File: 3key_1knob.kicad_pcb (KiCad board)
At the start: 2 copper layers, 17 parts, among them SW1 RotaryEncoder_Switch, U4 Kailh_socket_MX, U5 Kailh_socket_MX, U6 Kailh_socket_MX

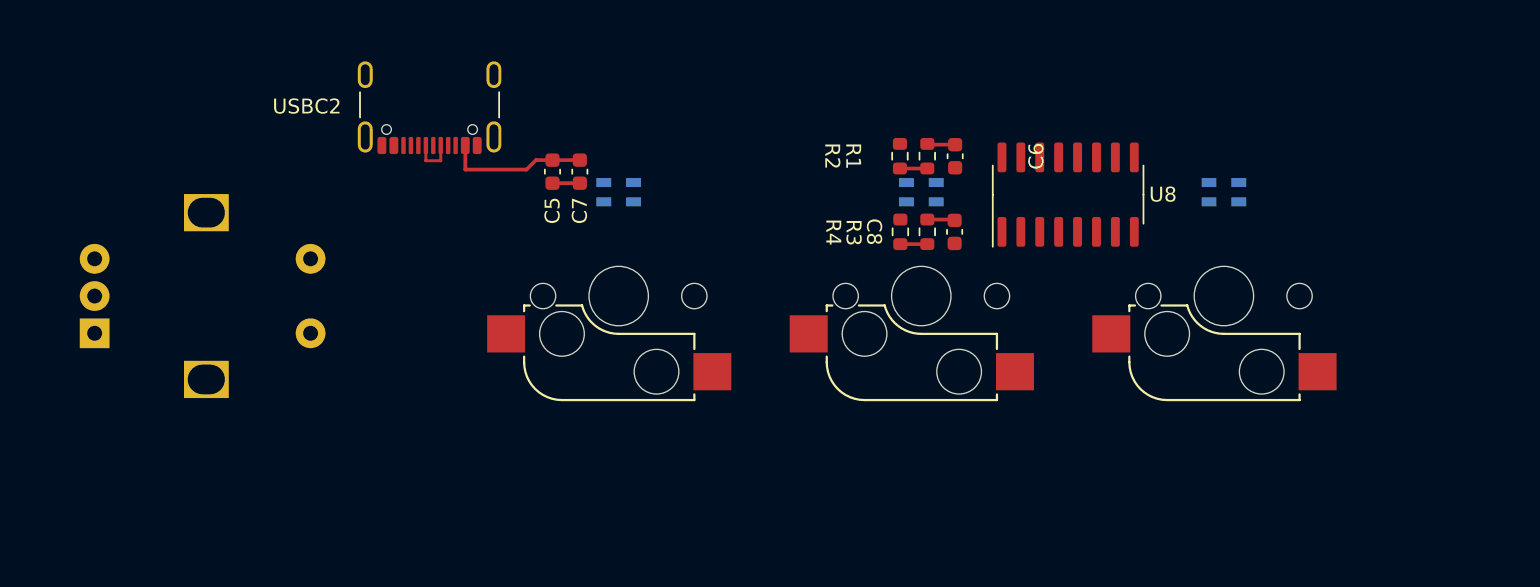
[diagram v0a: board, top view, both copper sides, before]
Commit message: Update PCB
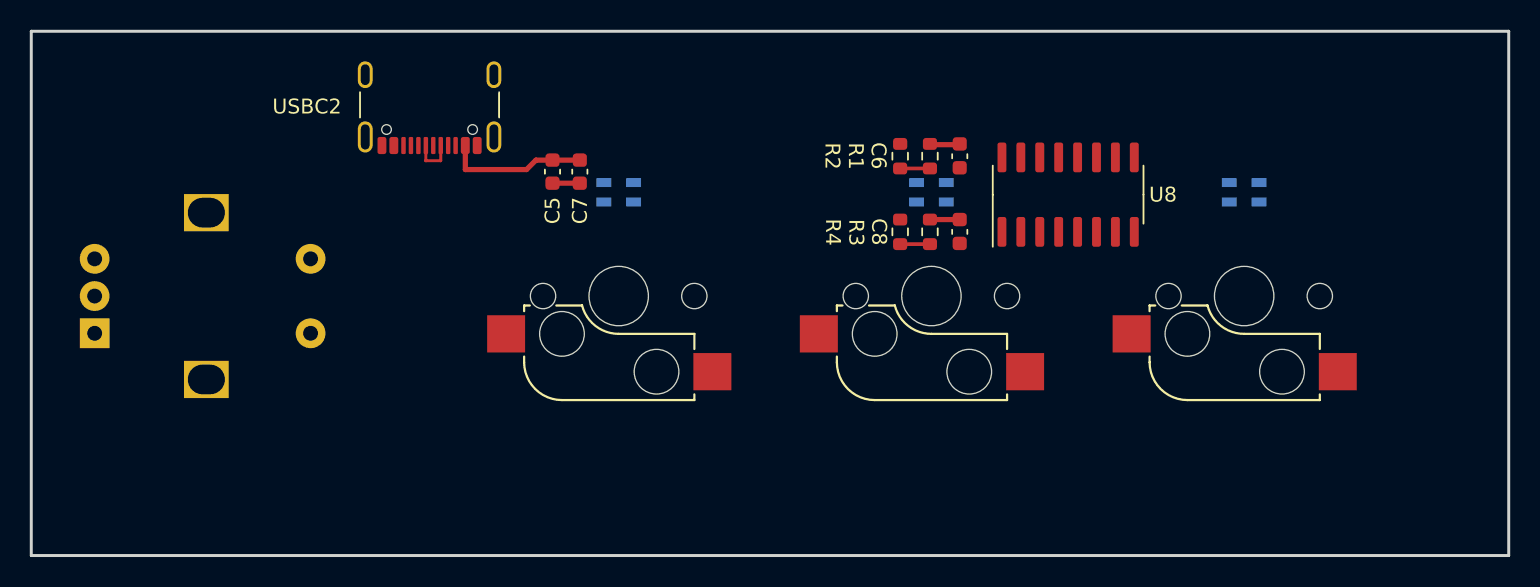
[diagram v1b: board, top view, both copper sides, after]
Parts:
- moved D3 1.36 mm to (130.9, 61.6)
- moved U4 1.36 mm to (130.9, 68.6)
- moved D2 0.68 mm to (109.9, 61.6)
- moved U5 0.68 mm to (109.9, 68.6)
- moved C8 0.34 mm to (111.8, 64.3)
- moved C6 0.31 mm to (111.8, 59.2)
- moved R1 0.18 mm to (109.8, 59.2)
- moved R3 0.18 mm to (109.8, 64.3)
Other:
- board outline added: 99.2 x 35.2 mm
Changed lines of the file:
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@@
   )
   (setup
+    (stackup
+      (layer "F.SilkS" (type "Top Silk Screen"))
+      (layer "F.Paste" (type "Top Solder Paste"))
+      (layer "F.Mask" (type "Top Solder Mask") (thickness 0.01))
+      (layer "F.Cu" (type "copper") (thickness 0.035))
+      (layer "dielectric 1" (type "core") (thickness 1.51) (material "FR4") (epsilon_r 4.5) (loss_tangent 0.02))
+      (layer "B.Cu" (type "copper") (thickness 0.035))
+      (layer "B.Mask" (type "Bottom Solder Mask") (thickness 0.01))
+      (layer "B.Paste" (type "Bottom Solder Paste"))
+      (layer "B.SilkS" (type "Bottom Silk Screen"))
+      (copper_finish "None")
+      (dielectric_constraints no)
+    )
     (pad_to_mask_clearance 0)
     (pcbplotparams
@@
   (net 26 "unconnected-(USBC2-CC1-PadA5)")
   (footprint "Resistor_SMD:R_0603_1608Metric" (layer "F.Cu")
-    (at 107.81542 64.268145 90)
+    (at 107.8 64.268145 90)
     (descr "Resistor SMD 0603 (1608 Metric), square (rectangular) end terminal, IPC_7351 nominal, (Body size source: IPC-SM-782 page 72, https://www.pcb-3d.com/wordpress/wp-content/uploads/ipc-sm-782a_amendment_1_and_2.pdf), generated with kicad-footprint-generator")
     (tags "resistor")
@@
   )
   (footprint "Resistor_SMD:R_0603_1608Metric" (layer "F.Cu")
-    (at 109.621682 59.187616 -90)
+    (at 109.8 59.187616 -90)
     (descr "Resistor SMD 0603 (1608 Metric), square (rectangular) end terminal, IPC_7351 nominal, (Body size source: IPC-SM-782 page 72, https://www.pcb-3d.com/wordpress/wp-content/uploads/ipc-sm-782a_amendment_1_and_2.pdf), generated with kicad-footprint-generator")
     (tags "resistor")
@@
     (fp_line (start 0.8 0.4125) (end -0.8 0.4125)
       (stroke (width 0.1) (type solid)) (layer "F.Fab"))
-    (pad "1" smd roundrect (at -0.825 0 270) (size 0.8 0.95) (layers "F.Cu" "F.Paste" "F.Mask") (roundrect_rratio 0.25)
+    (pad "1" smd roundrect (at -0.824471 0 270) (size 0.8 0.95) (layers "F.Cu" "F.Paste" "F.Mask") (roundrect_rratio 0.25)
       (net 3 "+3V3") (pintype "passive"))
     (pad "2" smd roundrect (at 0.825 0 270) (size 0.8 0.95) (layers "F.Cu" "F.Paste" "F.Mask") (roundrect_rratio 0.25)
@@
   )
   (footprint "Resistor_SMD:R_0603_1608Metric" (layer "F.Cu")
-    (at 109.621682 64.267616 -90)
+    (at 109.8 64.267616 -90)
     (descr "Resistor SMD 0603 (1608 Metric), square (rectangular) end terminal, IPC_7351 nominal, (Body size source: IPC-SM-782 page 72, https://www.pcb-3d.com/wordpress/wp-content/uploads/ipc-sm-782a_amendment_1_and_2.pdf), generated with kicad-footprint-generator")
     (tags "resistor")
@@
     (fp_line (start 0.8 0.4125) (end -0.8 0.4125)
       (stroke (width 0.1) (type solid)) (layer "F.Fab"))
-    (pad "1" smd roundrect (at -0.825 0 270) (size 0.8 0.95) (layers "F.Cu" "F.Paste" "F.Mask") (roundrect_rratio 0.25)
+    (pad "1" smd roundrect (at -0.824471 0 270) (size 0.8 0.95) (layers "F.Cu" "F.Paste" "F.Mask") (roundrect_rratio 0.25)
       (net 1 "+5V") (pintype "passive"))
     (pad "2" smd roundrect (at 0.825 0 270) (size 0.8 0.95) (layers "F.Cu" "F.Paste" "F.Mask") (roundrect_rratio 0.25)
@@
   )
   (footprint "Capacitor_SMD:C_0603_1608Metric" (layer "F.Cu")
-    (at 111.459538 64.270534 -90)
+    (at 111.8 64.270534 -90)
     (descr "Capacitor SMD 0603 (1608 Metric), square (rectangular) end terminal, IPC_7351 nominal, (Body size source: IPC-SM-782 page 76, https://www.pcb-3d.com/wordpress/wp-content/uploads/ipc-sm-782a_amendment_1_and_2.pdf), generated with kicad-footprint-generator")
     (tags "capacitor")
@@
     (fp_line (start 0.8 0.4) (end -0.8 0.4)
       (stroke (width 0.1) (type solid)) (layer "F.Fab"))
-    (pad "1" smd roundrect (at -0.775 0 270) (size 0.9 0.95) (layers "F.Cu" "F.Paste" "F.Mask") (roundrect_rratio 0.25)
+    (pad "1" smd roundrect (at -0.827389 0 270) (size 0.9 0.95) (layers "F.Cu" "F.Paste" "F.Mask") (roundrect_rratio 0.25)
       (net 1 "+5V") (pintype "passive"))
     (pad "2" smd roundrect (at 0.775 0 270) (size 0.9 0.95) (layers "F.Cu" "F.Paste" "F.Mask") (roundrect_rratio 0.25)
@@
   )
   (footprint "Capacitor_SMD:C_0603_1608Metric" (layer "F.Cu")
-    (at 111.494597 59.191526 -90)
+    (at 111.8 59.191526 -90)
     (descr "Capacitor SMD 0603 (1608 Metric), square (rectangular) end terminal, IPC_7351 nominal, (Body size source: IPC-SM-782 page 76, https://www.pcb-3d.com/wordpress/wp-content/uploads/ipc-sm-782a_amendment_1_and_2.pdf), generated with kicad-footprint-generator")
     (tags "capacitor")
@@
     (property "ki_keywords" "capacitor cap")
     (attr smd)
-    (fp_text reference "C6" (at -0.002009 -5.455995 90 unlocked) (layer "F.SilkS")
+    (fp_text reference "C6" (at -0.034926 5.449597 -90 unlocked) (layer "F.SilkS")
         (effects (font (size 1 1) (thickness 0.15)))
     )
@@
     (fp_line (start 0.8 0.4) (end -0.8 0.4)
       (stroke (width 0.1) (type solid)) (layer "F.Fab"))
-    (pad "1" smd roundrect (at -0.775 0 270) (size 0.9 0.95) (layers "F.Cu" "F.Paste" "F.Mask") (roundrect_rratio 0.25)
+    (pad "1" smd roundrect (at -0.828381 0 270) (size 0.9 0.95) (layers "F.Cu" "F.Paste" "F.Mask") (roundrect_rratio 0.25)
       (net 3 "+3V3") (pintype "passive"))
     (pad "2" smd roundrect (at 0.775 0 270) (size 0.9 0.95) (layers "F.Cu" "F.Paste" "F.Mask") (roundrect_rratio 0.25)
@@
   )
   (footprint "Resistor_SMD:R_0603_1608Metric" (layer "F.Cu")
-    (at 107.78542 59.188145 90)
+    (at 107.8 59.188145 90)
     (descr "Resistor SMD 0603 (1608 Metric), square (rectangular) end terminal, IPC_7351 nominal, (Body size source: IPC-SM-782 page 72, https://www.pcb-3d.com/wordpress/wp-content/uploads/ipc-sm-782a_amendment_1_and_2.pdf), generated with kicad-footprint-generator")
     (tags "resistor")
@@
   )
   (footprint "keyswitches:Kailh_socket_MX" (layer "B.Cu")
-    (at 109.22 68.58)
+    (at 109.9 68.58)
     (descr "MX-style keyswitch with Kailh socket mount")
     (tags "MX,cherry,gateron,kailh,pg1511,socket")
@@
   )
   (footprint "LED_SMD:LED_SK6805_PLCC4_2.4x2.7mm_P1.3mm" (layer "B.Cu")
-    (at 88.899999 61.61 180)
+    (at 88.9 61.61 180)
     (descr "https://cdn-shop.adafruit.com/product-files/3484/3484_Datasheet.pdf")
     (tags "LED RGB NeoPixel Nano PLCC-4")
@@
   )
   (footprint "keyswitches:Kailh_socket_MX" (layer "B.Cu")
-    (at 129.54 68.58)
+    (at 130.9 68.58)
     (descr "MX-style keyswitch with Kailh socket mount")
     (tags "MX,cherry,gateron,kailh,pg1511,socket")
@@
   )
   (footprint "LED_SMD:LED_SK6805_PLCC4_2.4x2.7mm_P1.3mm" (layer "B.Cu")
-    (at 109.219999 61.61 180)
+    (at 109.9 61.61 180)
     (descr "https://cdn-shop.adafruit.com/product-files/3484/3484_Datasheet.pdf")
     (tags "LED RGB NeoPixel Nano PLCC-4")
@@
   )
   (footprint "LED_SMD:LED_SK6805_PLCC4_2.4x2.7mm_P1.3mm" (layer "B.Cu")
-    (at 129.539999 61.61 180)
+    (at 130.9 61.61 180)
     (descr "https://cdn-shop.adafruit.com/product-files/3484/3484_Datasheet.pdf")
     (tags "LED RGB NeoPixel Nano PLCC-4")
@@
     )
   )
-  (gr_line (start 49.46 50.8) (end 148.66 50.8)
-    (stroke (width 0.2) (type default)) (layer "Dwgs.User"))
-  (gr_line (start 49.46 86) (end 148.66 86)
-    (stroke (width 0.2) (type default)) (layer "Dwgs.User"))
-  (gr_line (start 49.46 50.8) (end 49.46 86)
-    (stroke (width 0.2) (type default)) (layer "Dwgs.User"))
-  (gr_line (start 148.66 50.8) (end 148.66 86)
-    (stroke (width 0.2) (type default)) (layer "Dwgs.User"))
-  (segment (start 83.344924 59.451229) (end 84.454612 59.451229) (width 0.25) (layer "F.Cu") (net 1))
-  (segment (start 78.6 60.086982) (end 82.709171 60.086982) (width 0.25) (layer "F.Cu") (net 1))
-  (segment (start 82.709171 60.086982) (end 83.344924 59.451229) (width 0.25) (layer "F.Cu") (net 1))
-  (segment (start 84.454612 59.451229) (end 86.289127 59.451229) (width 0.25) (layer "F.Cu") (net 1))
-  (segment (start 78.6 58.472014) (end 78.6 60.086982) (width 0.25) (layer "F.Cu") (net 1))
+  (gr_rect (start 49.4538 50.8) (end 148.6662 86.0044)
+    (stroke (width 0.2) (type solid)) (fill none) (layer "Edge.Cuts"))
+  (segment (start 83.344924 59.451229) (end 84.454612 59.451229) (width 0.35) (layer "F.Cu") (net 1))
+  (segment (start 78.6 60.086982) (end 82.709171 60.086982) (width 0.35) (layer "F.Cu") (net 1))
+  (segment (start 82.709171 60.086982) (end 83.344924 59.451229) (width 0.35) (layer "F.Cu") (net 1))
+  (segment (start 84.454612 59.451229) (end 86.289127 59.451229) (width 0.35) (layer "F.Cu") (net 1))
+  (segment (start 78.6 58.472014) (end 78.6 60.086982) (width 0.35) (layer "F.Cu") (net 1))
   (segment (start 111.40662 63.442616) (end 111.459538 63.495534) (width 0.25) (layer "F.Cu") (net 1))
   (segment (start 86.289127 59.451229) (end 86.289535 59.451637) (width 0.25) (layer "F.Cu") (net 1))
-  (segment (start 109.621682 63.442616) (end 111.40662 63.442616) (width 0.25) (layer "F.Cu") (net 1))
+  (segment (start 109.621682 63.442616) (end 111.40662 63.442616) (width 0.35) (layer "F.Cu") (net 1))
   (segment (start 84.45502 61.001637) (end 84.454612 61.001229) (width 0.25) (layer "F.Cu") (net 2))
-  (segment (start 86.289535 61.001637) (end 84.45502 61.001637) (width 0.25) (layer "F.Cu") (net 2))
-  (segment (start 111.51405 58.414997) (end 109.674063 58.414997) (width 0.25) (layer "F.Cu") (net 3))
+  (segment (start 86.289535 61.001637) (end 84.45502 61.001637) (width 0.35) (layer "F.Cu") (net 2))
+  (segment (start 111.51405 58.414997) (end 109.674063 58.414997) (width 0.35) (layer "F.Cu") (net 3))
   (segment (start 109.674063 58.414997) (end 109.621682 58.362616) (width 0.25) (layer "F.Cu") (net 3))
   (segment (start 76.95 59.492373) (end 76.949367 59.493006) (width 0.2) (layer "F.Cu") (net 9))

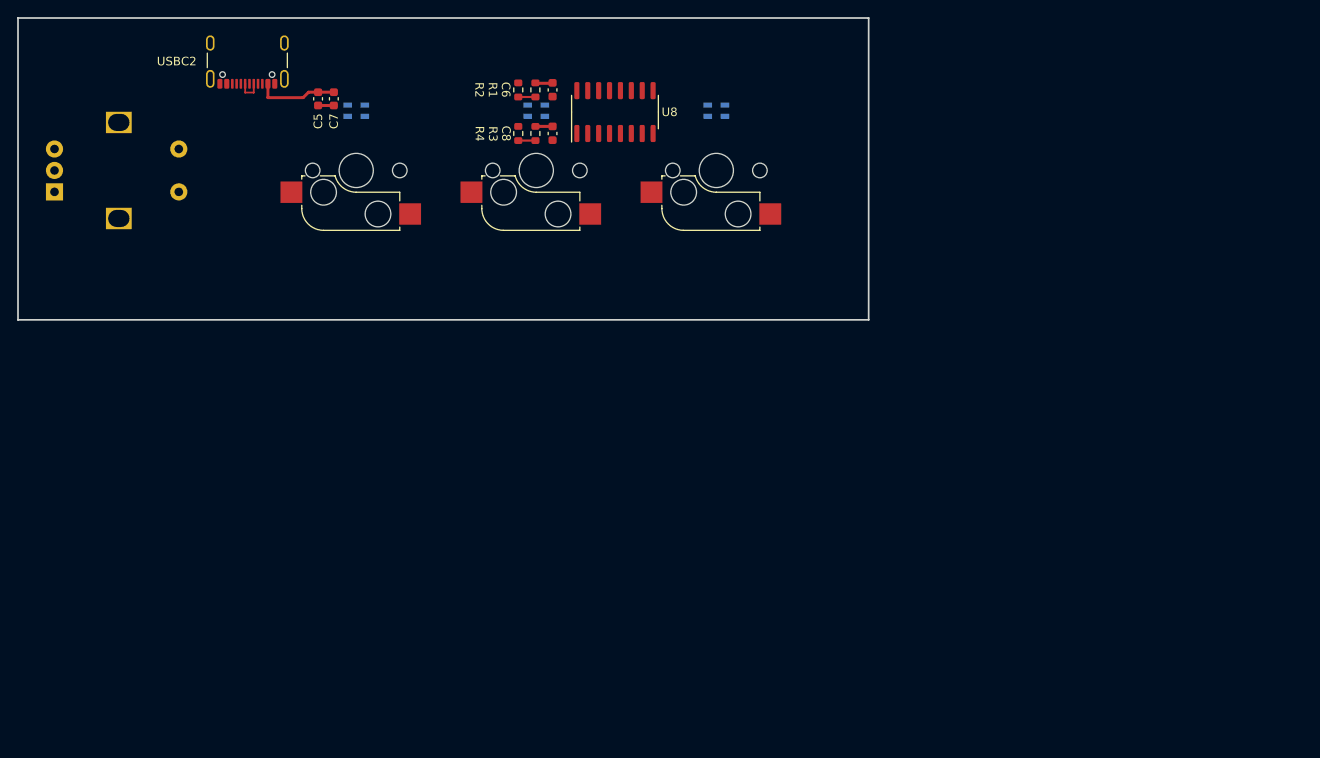
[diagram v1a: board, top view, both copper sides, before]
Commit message: Unrouted PCB
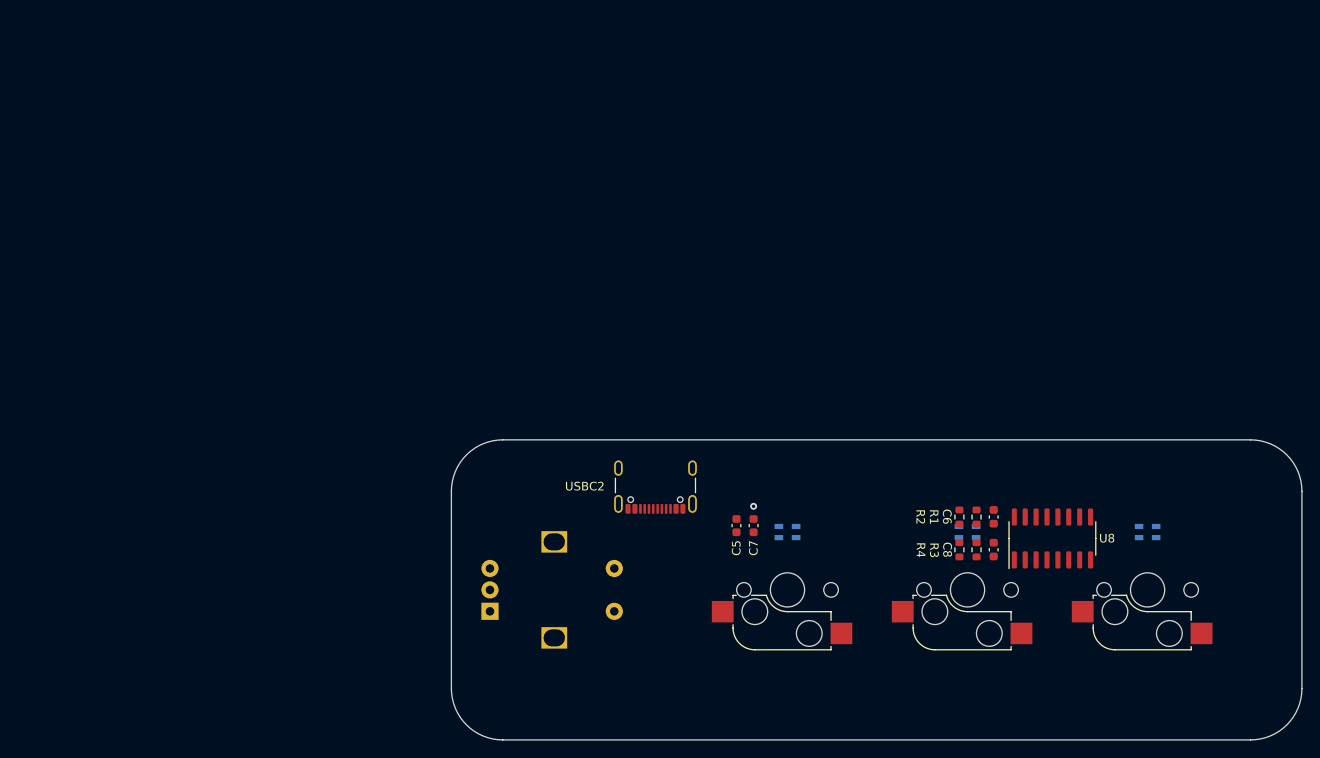
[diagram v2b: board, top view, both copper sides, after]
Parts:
- moved R1 71.6 mm to (161.2, 109.0)
- moved R2 71.6 mm to (159.2, 109.0)
- moved C6 71.6 mm to (163.2, 109.0)
- moved U8 71.2 mm to (170.1, 111.5)
- moved R3 70.7 mm to (161.2, 112.8)
- moved R4 70.7 mm to (159.2, 112.8)
- moved C8 70.7 mm to (163.2, 112.8)
- moved SW1 70.5 mm to (104.5, 120.0)
- moved D1 70.3 mm to (139.2, 110.8)
- moved D2 70.3 mm to (160.2, 110.8)
- moved D3 70.3 mm to (181.2, 110.8)
- moved U4 70.2 mm to (181.2, 117.5)
- moved U5 70.2 mm to (160.2, 117.5)
- moved U6 70.2 mm to (139.2, 117.5)
- moved C7 69.8 mm to (135.2, 110.0)
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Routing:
- net +5V: track 11.4 -> 0.00 mm, vias 0 -> 1
- net /D-: track 3.04 -> 0.00 mm
- net +3V3: track 1.91 -> 0.00 mm
- net Net-(R1-Pad2): track 1.84 -> 0.00 mm
- net GND: track 1.84 -> 0.00 mm
- net /LED_DO: track 1.81 -> 0.00 mm
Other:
- board size 99.2 x 35.2 mm -> 99.2 x 35 mm
